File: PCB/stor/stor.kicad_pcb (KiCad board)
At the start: 4 copper layers, 22 x 60.5 mm, 58 parts, among them J1 Conn_01x05_Socket, J2 Conn_01x04_Socket, SW1 TS1603-TZ38HBM, SW2 TS1603-TZ38HBM, U1 STM32H723VGT6, U3 USB3300-EZK-TR, U4 TPS62177DQCR, X1 25mhz, X2 32.768k, X3 24mhz

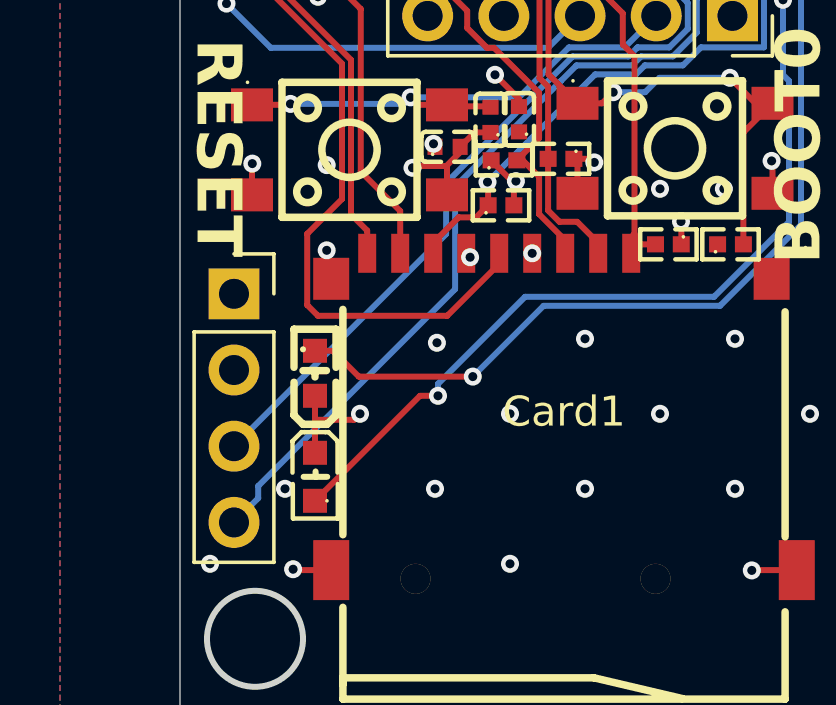
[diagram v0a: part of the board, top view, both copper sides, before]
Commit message: tt
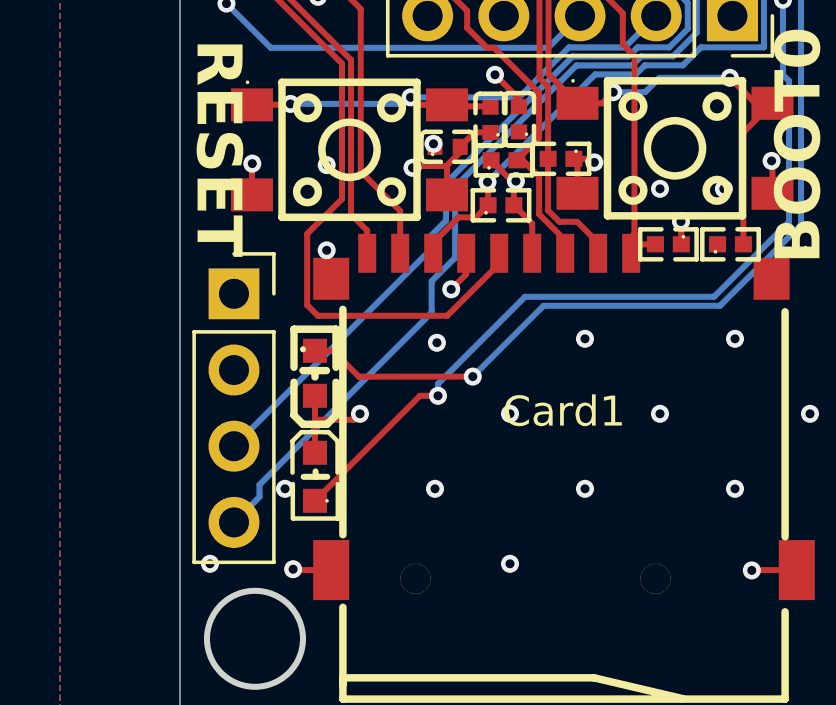
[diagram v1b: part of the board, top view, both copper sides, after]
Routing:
- net /VDD: track 54.9 -> 56.7 mm, vias 25 -> 24
- net GND: track 73.3 -> 74.7 mm
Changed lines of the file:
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@@
 	)
 	(segment
+		(start 120.74 78.66)
+		(end 120.74 79.65)
+		(width 0.2)
+		(layer "F.Cu")
+		(net "/VDD")
+	)
+	(segment
 		(start 125 64.1)
 		(end 125 65.1)
@@
 	)
 	(segment
+		(start 120.13 78.05)
+		(end 120.74 78.66)
+		(width 0.2)
+		(layer "F.Cu")
+		(net "/VDD")
+	)
+	(segment
 		(start 113.75 50)
 		(end 114.275997 50)
@@
 	)
 	(via
-		(at 120.74 79.65)
-		(size 0.6)
-		(drill 0.3)
-		(layers "F.Cu" "B.Cu")
-		(net "/VDD")
-	)
-	(via
 		(at 111.14 40.76)
 		(size 0.6)
@@
 	)
 	(segment
+		(start 118.54 79.65)
+		(end 118.54 80.35)
+		(width 0.2)
+		(layer "F.Cu")
+		(net "GND")
+	)
+	(segment
 		(start 128.25 49.77)
 		(end 128.25 50.16)
@@
 	)
 	(segment
+		(start 118.54 80.35)
+		(end 118.04 80.85)
+		(width 0.2)
+		(layer "F.Cu")
+		(net "GND")
+	)
+	(segment
 		(start 120.2 43.25)
 		(end 121.1 44.15)
@@
 	)
 	(via
-		(at 118.66962 79.77962)
-		(size 0.6)
-		(drill 0.3)
-		(layers "F.Cu" "B.Cu")
-		(net "GND")
-	)
-	(via
 		(at 128.84 45.400002)
 		(size 0.6)
@@
 	)
 	(via
+		(at 118.04 80.85)
+		(size 0.6)
+		(drill 0.3)
+		(layers "F.Cu" "B.Cu")
+		(net "GND")
+	)
+	(via
 		(at 120 90)
 		(size 0.6)
@@
 	)
 	(segment
-		(start 125.309925 72.785)
-		(end 125.925 72.169925)
+		(start 117.9 52.819239)
+		(end 117.145778 52.065017)
+		(width 0.2)
+		(layer "B.Cu")
+		(net "/PA9")
+	)
+	(segment
+		(start 117.9 54.024264)
+		(end 117.9 52.819239)
 		(width 0.2)
 		(layer "B.Cu")
@@
 	)
 	(segment
-		(start 122.088736 73.087)
-		(end 123.947264 73.087)
+		(start 125.134189 61.258453)
+		(end 117.9 54.024264)
 		(width 0.2)
 		(layer "B.Cu")
@@
 	)
 	(segment
-		(start 117.86962 77.306116)
-		(end 122.088736 73.087)
+		(start 117.86962 78.556877)
+		(end 117.86962 77.306116)
 		(width 0.2)
 		(layer "B.Cu")
@@
 	)
 	(segment
-		(start 125.134189 61.258453)
-		(end 117.9 54.024264)
+		(start 123.947264 73.087)
+		(end 124.249265 72.785)
 		(width 0.2)
 		(layer "B.Cu")
@@
 	)
 	(segment
-		(start 117.9 52.819239)
-		(end 117.145778 52.065017)
+		(start 117.28 79.6)
+		(end 117.28 79.146497)
 		(width 0.2)
 		(layer "B.Cu")
@@
 	)
 	(segment
-		(start 125.925 71.300075)
-		(end 125.134189 70.509264)
+		(start 117.86962 77.306116)
+		(end 122.088736 73.087)
 		(width 0.2)
 		(layer "B.Cu")
@@
 	)
 	(segment
-		(start 117.86962 79.01038)
-		(end 117.86962 77.306116)
+		(start 125.309925 72.785)
+		(end 125.925 72.169925)
 		(width 0.2)
 		(layer "B.Cu")
@@
 	)
 	(segment
-		(start 117.9 54.024264)
-		(end 117.9 52.819239)
+		(start 110.8 86.08)
+		(end 117.28 79.6)
 		(width 0.2)
 		(layer "B.Cu")
@@
 	)
 	(segment
-		(start 123.947264 73.087)
-		(end 124.249265 72.785)
+		(start 117.28 79.146497)
+		(end 117.86962 78.556877)
 		(width 0.2)
 		(layer "B.Cu")
@@
 	)
 	(segment
-		(start 110.8 86.08)
-		(end 117.86962 79.01038)
+		(start 125.925 71.300075)
+		(end 125.134189 70.509264)
+		(width 0.2)
+		(layer "B.Cu")
+		(net "/PA9")
+	)
+	(segment
+		(start 122.088736 73.087)
+		(end 123.947264 73.087)
 		(width 0.2)
 		(layer "B.Cu")
@@
 	)
 	(segment
-		(start 122.215828 73.387)
-		(end 124.071528 73.387)
+		(start 118.16962 79.801141)
+		(end 118.16962 77.43038)
 		(width 0.2)
 		(layer "B.Cu")
@@
 	)
 	(segment
-		(start 125.434189 61.134189)
-		(end 118.2 53.9)
+		(start 122.215828 73.387)
+		(end 124.071528 73.387)
 		(width 0.2)
 		(layer "B.Cu")
@@
 	)
 	(segment
-		(start 111.607463 87.812537)
-		(end 110.8 88.62)
+		(start 125.434189 61.134189)
+		(end 118.2 53.9)
 		(width 0.2)
 		(layer "B.Cu")
@@
 	)
 	(segment
-		(start 111.607463 87.407463)
-		(end 118.16962 80.845305)
+		(start 117.39 80.580761)
+		(end 118.16962 79.801141)
 		(width 0.2)
 		(layer "B.Cu")
@@
 	)
 	(segment
-		(start 118.16962 77.43038)
-		(end 121.7 73.9)
+		(start 111.65 87.364925)
+		(end 117.39 81.624925)
 		(width 0.2)
 		(layer "B.Cu")
@@
 	)
 	(segment
+		(start 117.39 81.624925)
+		(end 117.39 80.580761)
+		(width 0.2)
+		(layer "B.Cu")
+		(net "/PA10")
+	)
+	(segment
 		(start 126.225 71.175811)
 		(end 125.434189 70.385)
@@
 	)
 	(segment
-		(start 118.16962 80.845305)
-		(end 118.16962 77.43038)
+		(start 110.8 88.62)
+		(end 111.65 87.77)
 		(width 0.2)
 		(layer "B.Cu")
@@
 	)
 	(segment
-		(start 118.2 53.9)
-		(end 118.2 52)
+		(start 111.65 87.77)
+		(end 111.65 87.364925)
+		(width 0.2)
+		(layer "B.Cu")
+		(net "/PA10")
+	)
+	(segment
+		(start 118.16962 77.43038)
+		(end 121.7 73.9)
 		(width 0.2)
 		(layer "B.Cu")
@@
 	)
 	(segment
-		(start 111.607463 87.407463)
-		(end 111.607463 87.812537)
+		(start 118.2 53.9)
+		(end 118.2 52)
 		(width 0.2)
 		(layer "B.Cu")
